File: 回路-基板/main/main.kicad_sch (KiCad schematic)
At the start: 5 parts, among them J1 Conn_01x02_Pin, U1 TWE-L-WX

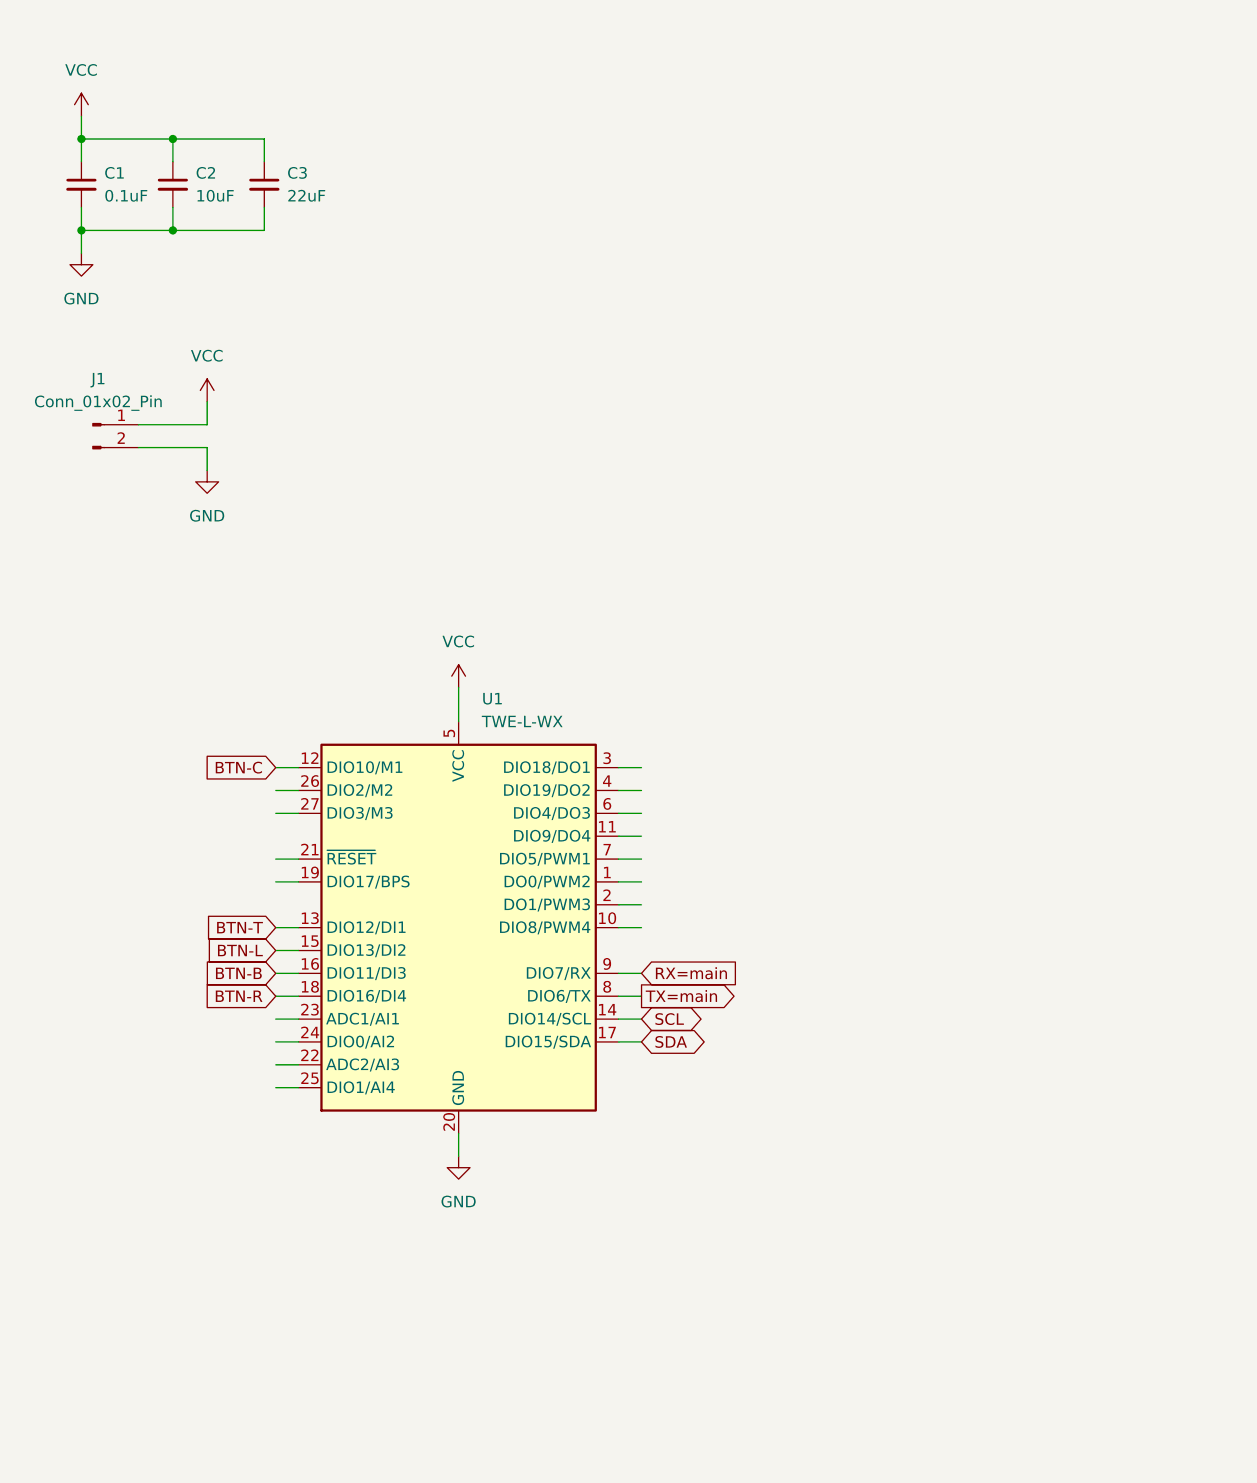
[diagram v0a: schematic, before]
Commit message: 回路やったぜぇ
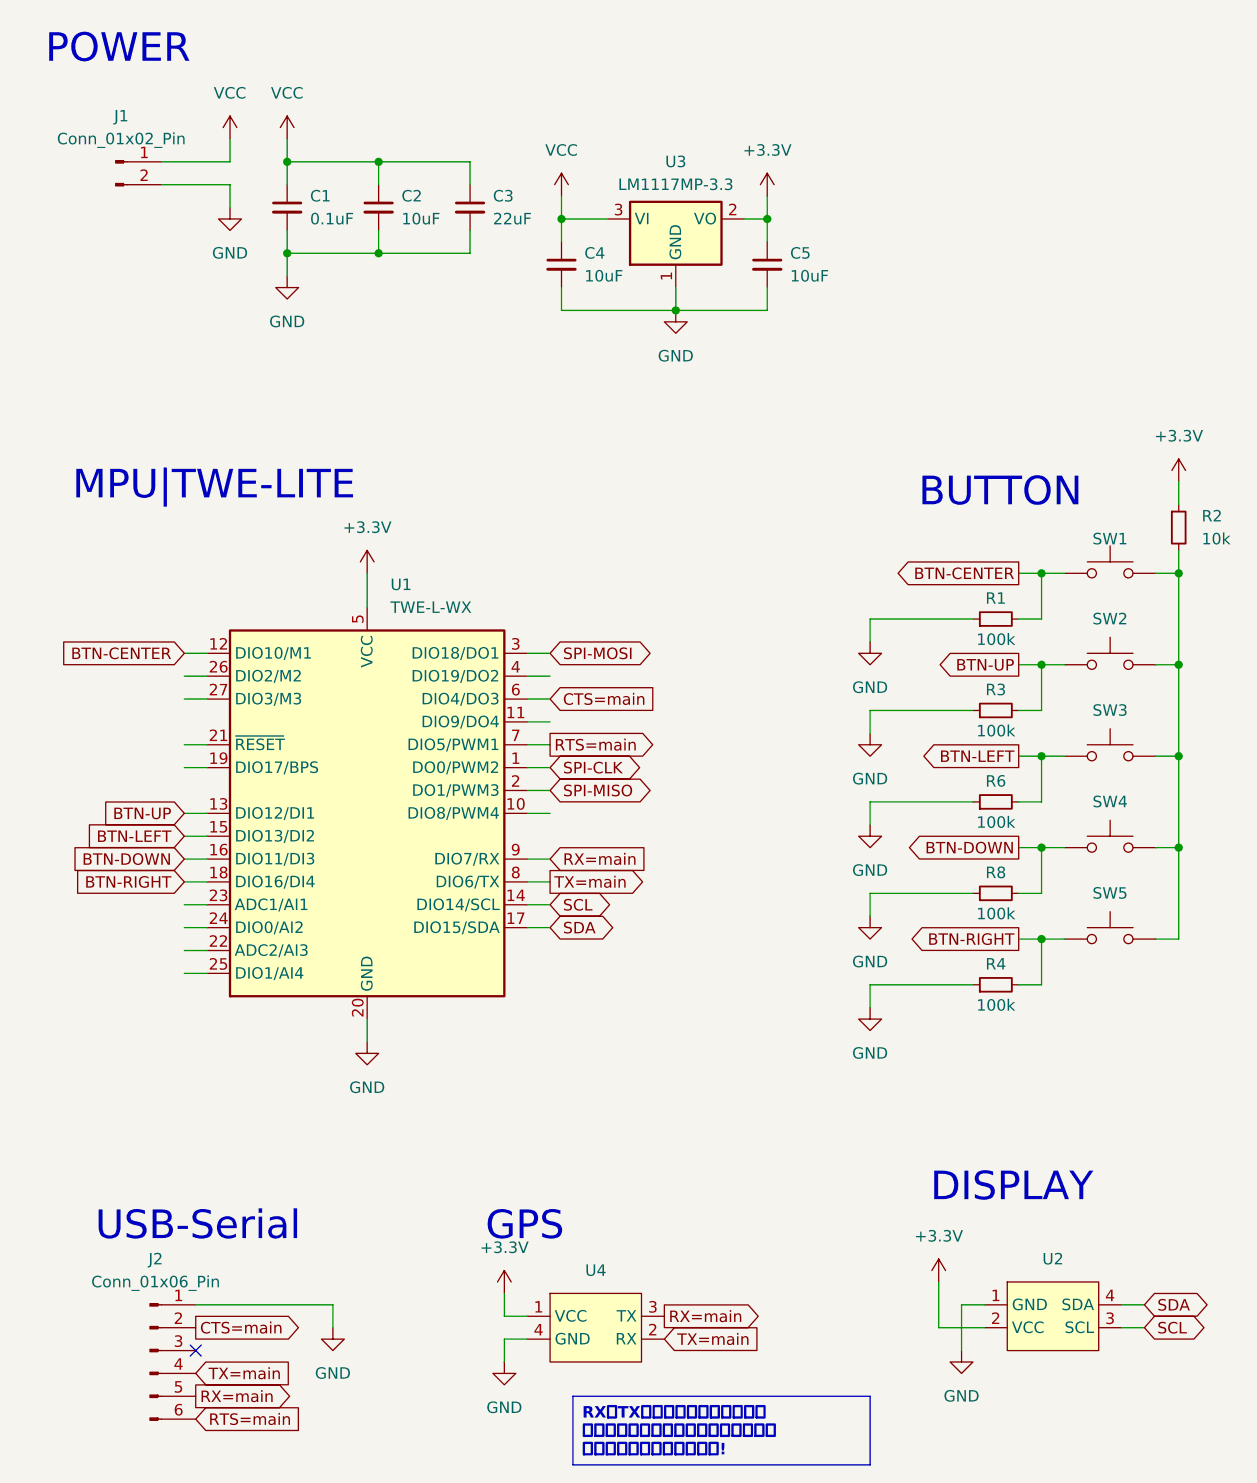
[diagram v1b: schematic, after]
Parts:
- added C4, C5: 10uF, symbol Device:C_Small
- added J2: Conn_01x06_Pin, symbol Connector:Conn_01x06_Pin
- added R1, R3, R4, R6, R8: 100k, symbol Device:R_Small
- added R2: 10k, symbol Device:R_Small
- added SW1, SW2, SW3, SW4, SW5: SW_Push, symbol Switch:SW_Push
- added U2: ~, symbol CanSat:Display-I2C
- added U3: LM1117MP-3.3, Package_TO_SOT_SMD:SOT-223-3_TabPin2, symbol Regulator_Linear:LM1117MP-3.3
- added U4: ~, symbol CanSat:GY-NEO6MV2
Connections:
- net GND: now also C4.2, C5.2, J2.1 (Pin_1), R1.1, R3.1, R4.1, R6.1, R8.1, U2.1 (GND), U3.1 (GND), U4.4 (GND)
- net RX=main: now also J2.5 (Pin_5), U4.3 (TX)
- net SCL: now also U2.3 (SCL)
- net SDA: now also U2.4 (SDA)
- net TX=main: now also J2.4 (Pin_4), U4.2 (RX)
- net VCC: now also C4.1, U3.3 (VI); no longer U1.5 (VCC)
- net SPI-CLK: now reaches U1.1 (DO0/PWM2)
- net SPI-MISO: now reaches U1.2 (DO1/PWM3)
- net SPI-MOSI: now reaches U1.3 (DIO18/DO1)
- net CTS=main: now reaches U1.6 (DIO4/DO3)
- net CTS=main: now also J2.2 (Pin_2)
- net RTS=main: now reaches U1.7 (DIO5/PWM1)
- net RTS=main: now also J2.6 (Pin_6)
- net BTN-B renamed BTN-DOWN
- net BTN-DOWN: now also R8.2, SW4.1
- net BTN-C renamed BTN-CENTER
- net BTN-CENTER: now also R1.2, SW1.1
- net BTN-L renamed BTN-LEFT
- net BTN-LEFT: now also R6.2, SW3.1
- net BTN-R renamed BTN-RIGHT
- net BTN-RIGHT: now also R4.2, SW5.1
- net BTN-T renamed BTN-UP
- net BTN-UP: now also R3.2, SW2.1
- new net: R2.2, SW1.2, SW2.2, SW3.2, SW4.2, SW5.2
- new net +3.3V: C5.1, R2.1, U1.5 (VCC), U2.2 (VCC), U3.2 (VO), U4.1 (VCC)
- no-connect marks 0 -> 1
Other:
- note added: "BUTTON"
- note added: "DISPLAY"
- note added: "GPS"
- note added: "MPU|TWE-LITE"
- note added: "POWER"
- note added: "USB-Serial"
- moved on the sheet: C1, C2, C3, J1, U1
